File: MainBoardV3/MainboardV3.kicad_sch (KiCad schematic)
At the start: 31 parts, among them J1 Conn_01x02, J10 Conn_01x04, J11 Conn_01x02, J18 Conn_01x03, J19 Conn_02x03_Odd_Even, J2 Conn_01x04, J20 Conn_02x03_Odd_Even, J21 Conn_02x03_Odd_Even, J22 Conn_01x03, J23 Conn_01x05, J24 Conn_02x05_Odd_Even, J3 Conn_01x03, J4 Conn_01x04, J5 Conn_01x05, J7 Conn_01x04, J8 Conn_01x04, J9 Conn_01x04, U2 ESP32-S3-DevKitC

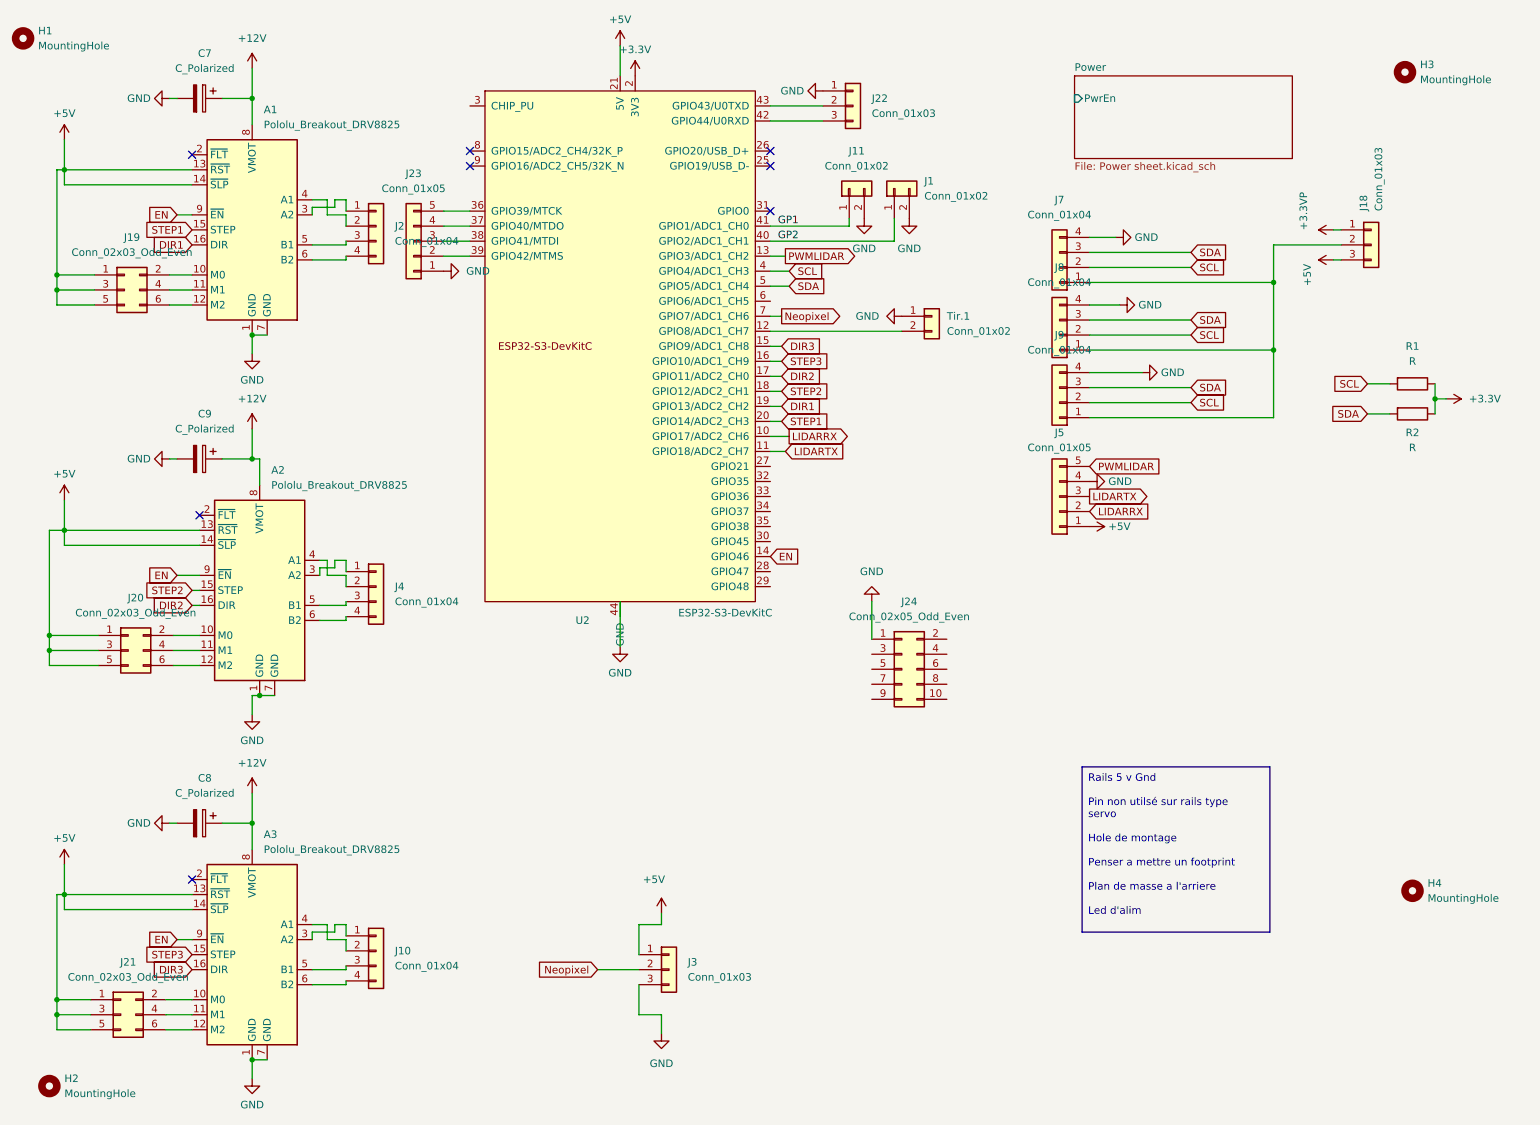
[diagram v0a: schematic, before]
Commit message: Mise a jour pour remi
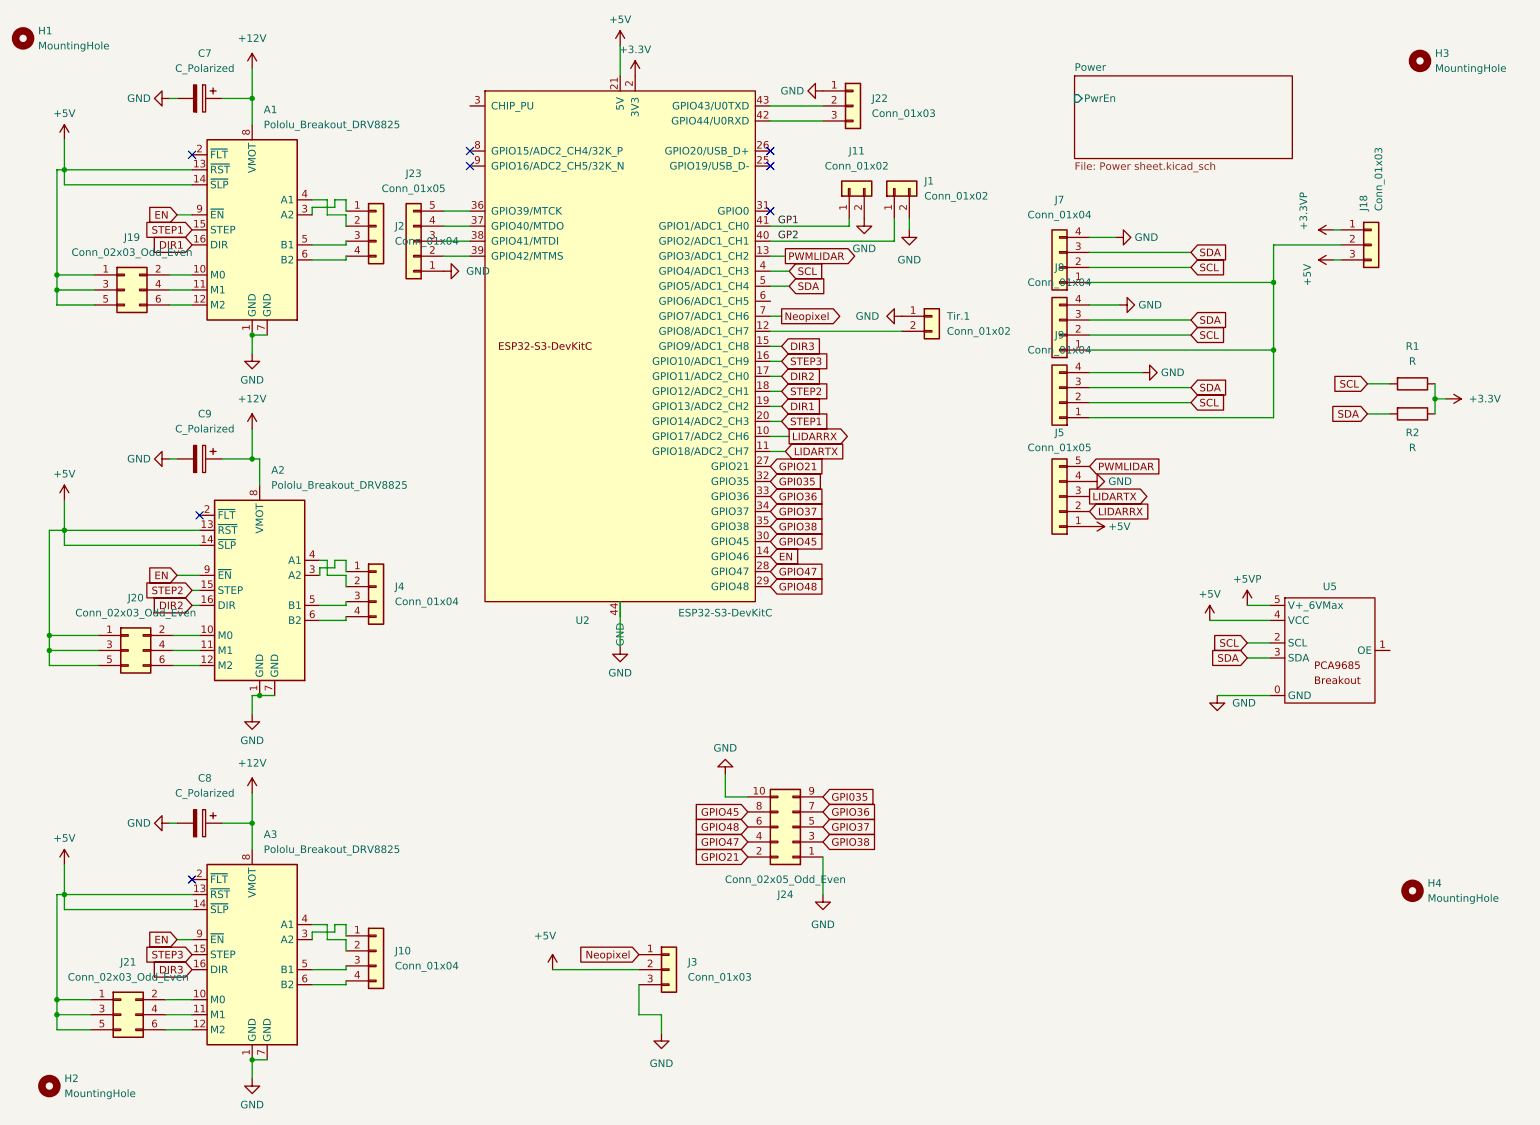
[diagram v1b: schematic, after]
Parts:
- added U5: ~, Custom:PCA9685breakout, symbol PCM:PWMI2C
- H1, H2, H3, H4: footprint MountingHole:MountingHole_3.2mm_M3_DIN965_Pad -> MountingHole:MountingHole_3.2mm_M3
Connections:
- net +5V: now also J3.2 (Pin_2), U5.4 (VCC); no longer J3.1 (Pin_1)
- net GND: now also J24.10 (Pin_10), U5.0 (GND)
- net Neopixel: now also J3.1 (Pin_1); no longer J3.2 (Pin_2)
- net SCL: now also U5.2 (SCL)
- net SDA: now also U5.3 (SDA)
- net GPIO21: now reaches J24.2 (Pin_2)
- net GPIO21: now also U2.27 (GPIO21)
- net GPIO38: now reaches J24.3 (Pin_3)
- net GPIO38: now also U2.35 (GPIO38)
- net GPIO47: now reaches J24.4 (Pin_4)
- net GPIO47: now also U2.28 (GPIO47)
- net GPIO37: now reaches J24.5 (Pin_5)
- net GPIO37: now also U2.34 (GPIO37)
- net GPIO48: now reaches J24.6 (Pin_6)
- net GPIO48: now also U2.29 (GPIO48)
- net GPIO36: now reaches J24.7 (Pin_7)
- net GPIO36: now also U2.33 (GPIO36)
- net GPIO45: now reaches J24.8 (Pin_8)
- net GPIO45: now also U2.30 (GPIO45)
- net GPI035: now reaches J24.9 (Pin_9)
- net GPI035: now also U2.32 (GPIO35)
- new net +5VP: U5.5 (V+_6VMax)
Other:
- moved on the sheet: H3, J24
